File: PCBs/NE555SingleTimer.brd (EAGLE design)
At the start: 22.5 x 32 mm, 5 parts, among them IC1 LM555N

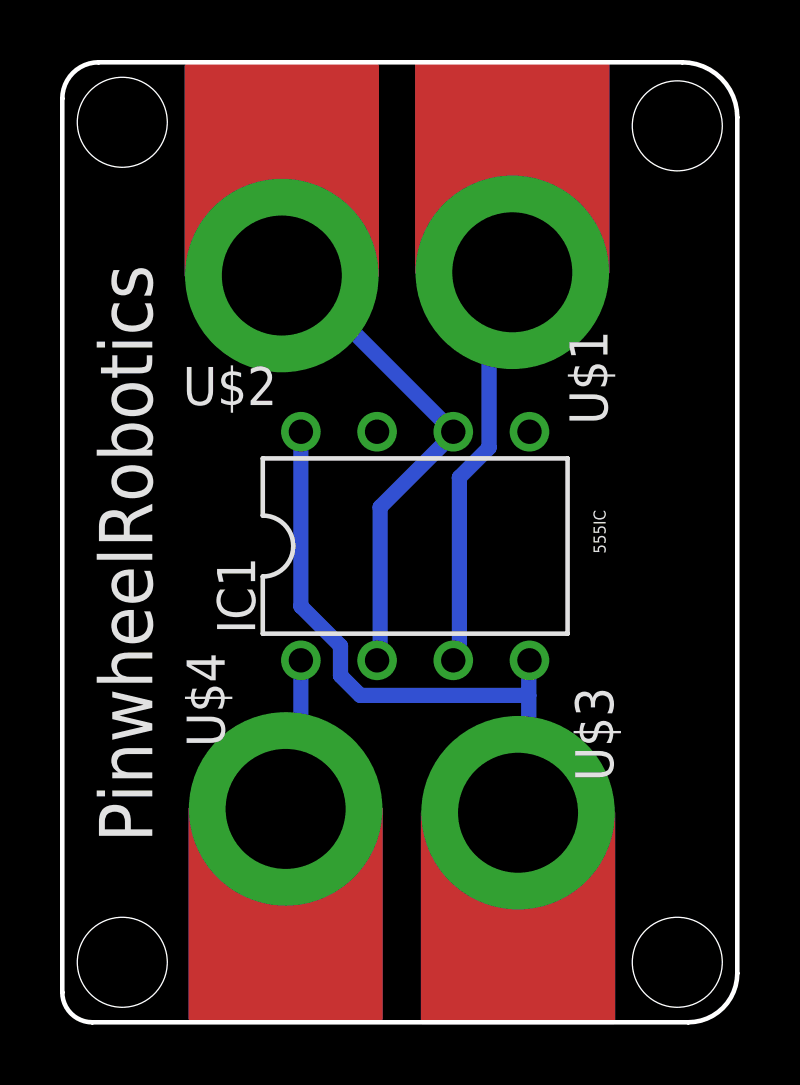
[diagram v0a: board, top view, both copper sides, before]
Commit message: New Update
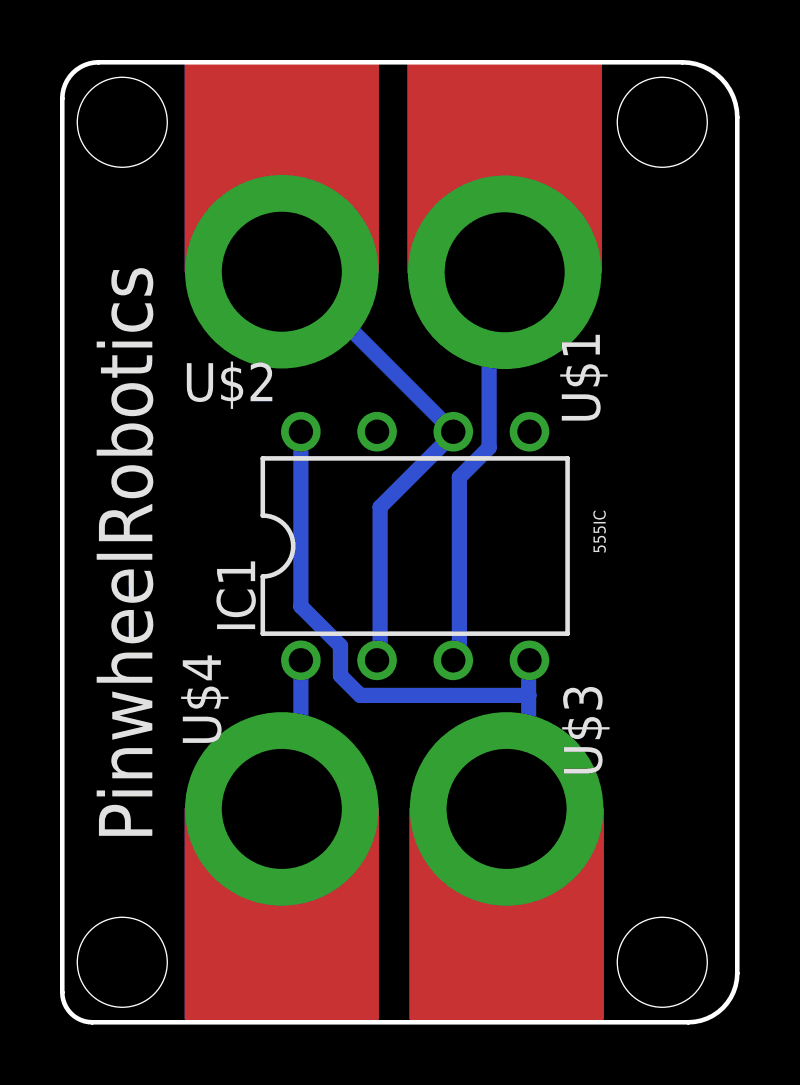
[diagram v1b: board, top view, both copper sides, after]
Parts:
- moved U$3 0.40 mm to (11.8, 7.11)
- moved U$1 0.25 mm to (11.7, 25.0)
- moved U$4 0.13 mm to (4.32, 7.11)
- moved U$2 0.13 mm to (4.32, 25.0)
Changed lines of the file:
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@@
 <drawing>
 <settings>
-<setting alwaysvectorfont="yes"/>
+<setting alwaysvectorfont="no"/>
 <setting verticaltext="up"/>
 </settings>
@@
 <wire x1="-1.788903125" y1="32" x2="-3" y2="30.788903125" width="0.1524" layer="20" curve="90"/>
 <hole x="-1" y="30" drill="3"/>
-<hole x="17.5" y="29.881" drill="3"/>
-<hole x="17.5" y="2" drill="3"/>
+<hole x="17" y="30" drill="3"/>
+<hole x="17" y="2" drill="3"/>
 <hole x="-1" y="2" drill="3"/>
 <text x="0" y="6" size="1.778" layer="21" rot="R90">PinwheelRobotics </text>
@@
 <attribute name="VALUE" x="5.207" y="15.24" size="1.27" layer="27" ratio="10"/>
 </element>
-<element name="U$1" library="microbit" package="MICROBIT_PAD" value="MICROBIT_PAD" x="12" y="25" smashed="yes" rot="R180">
-<attribute name="NAME" x="15.175" y="19.92" size="1.27" layer="21" rot="R90"/>
+<element name="U$1" library="microbit" package="MICROBIT_PAD" value="MICROBIT_PAD" x="11.746" y="25" smashed="yes" rot="R180">
+<attribute name="NAME" x="14.921" y="19.92" size="1.27" layer="21" rot="R90"/>
 </element>
-<element name="U$2" library="microbit" package="MICROBIT_PAD" value="MICROBIT_PAD" x="4.318" y="24.892" smashed="yes" rot="R180">
-<attribute name="NAME" x="1.016" y="20.574" size="1.27" layer="21"/>
+<element name="U$2" library="microbit" package="MICROBIT_PAD" value="MICROBIT_PAD" x="4.318" y="25.019" smashed="yes" rot="R180">
+<attribute name="NAME" x="1.016" y="20.701" size="1.27" layer="21"/>
 </element>
-<element name="U$3" library="microbit" package="MICROBIT_PAD" value="MICROBIT_PAD" x="12.192" y="6.985" smashed="yes">
-<attribute name="NAME" x="14.097" y="11.176" size="1.27" layer="21" rot="R270"/>
+<element name="U$3" library="microbit" package="MICROBIT_PAD" value="MICROBIT_PAD" x="11.811" y="7.112" smashed="yes">
+<attribute name="NAME" x="13.716" y="11.303" size="1.27" layer="21" rot="R270"/>
 </element>
-<element name="U$4" library="microbit" package="MICROBIT_PAD" value="MICROBIT_PAD" x="4.445" y="7.112" smashed="yes">
-<attribute name="NAME" x="1.143" y="12.319" size="1.27" layer="21" rot="R270"/>
+<element name="U$4" library="microbit" package="MICROBIT_PAD" value="MICROBIT_PAD" x="4.318" y="7.112" smashed="yes">
+<attribute name="NAME" x="1.016" y="12.319" size="1.27" layer="21" rot="R270"/>
 </element>
 </elements>
@@
 <wire x1="12.5476" y1="7.5946" x2="12.5476" y2="10.8966" width="0.508" layer="16"/>
 <wire x1="12.5476" y1="10.8966" x2="12.5476" y2="11.8872" width="0.508" layer="16"/>
-<wire x1="12.2428" y1="7.2898" x2="12.5476" y2="7.5946" width="0.508" layer="16"/>
+<wire x1="12.1158" y1="7.1628" x2="12.5476" y2="7.5946" width="0.508" layer="16"/>
 <wire x1="12.5476" y1="11.8872" x2="12.573" y2="12.065" width="0.508" layer="16"/>
-<wire x1="12.2428" y1="7.2898" x2="12.192" y2="6.985" width="0.508" layer="16"/>
+<wire x1="12.1158" y1="7.1628" x2="11.811" y2="7.112" width="0.508" layer="16"/>
 <wire x1="4.953" y1="13.8684" x2="4.953" y2="19.685" width="0.508" layer="16"/>
 <wire x1="6.2738" y1="12.5476" x2="4.953" y2="13.8684" width="0.508" layer="16"/>
@@
 <wire x1="11.2268" y1="19.1516" x2="10.2362" y2="18.161" width="0.508" layer="16"/>
 <wire x1="11.2268" y1="24.1046" x2="11.2268" y2="19.1516" width="0.508" layer="16"/>
-<wire x1="12" y1="24.8778" x2="11.2268" y2="24.1046" width="0.508" layer="16"/>
+<wire x1="11.746" y1="24.6238" x2="11.2268" y2="24.1046" width="0.508" layer="16"/>
 <wire x1="10.2362" y1="12.2174" x2="10.033" y2="12.065" width="0.508" layer="16"/>
-<wire x1="12" y1="24.8778" x2="12" y2="25" width="0.508" layer="16"/>
+<wire x1="11.746" y1="24.6238" x2="11.746" y2="25" width="0.508" layer="16"/>
 </signal>
 <signal name="N$2">
@@
 <wire x1="7.5946" y1="12.2174" x2="7.493" y2="12.065" width="0.508" layer="16"/>
 <wire x1="9.906" y1="19.4818" x2="10.033" y2="19.685" width="0.508" layer="16"/>
-<wire x1="4.826" y1="24.892" x2="10.033" y2="19.685" width="0.508" layer="16"/>
-<wire x1="4.318" y1="24.892" x2="4.826" y2="24.892" width="0.508" layer="16"/>
+<wire x1="4.699" y1="25.019" x2="10.033" y2="19.685" width="0.508" layer="16"/>
+<wire x1="4.318" y1="25.019" x2="4.699" y2="25.019" width="0.508" layer="16"/>
 </signal>
 <signal name="GND">
 <contactref element="IC1" pad="1"/>
 <contactref element="U$4" pad="PAD"/>
-<wire x1="4.953" y1="7.5946" x2="4.953" y2="12.065" width="0.508" layer="16"/>
-<wire x1="4.6228" y1="7.2644" x2="4.953" y2="7.5946" width="0.508" layer="16"/>
-<wire x1="4.6228" y1="7.2644" x2="4.445" y2="7.112" width="0.508" layer="16"/>
+<wire x1="4.953" y1="7.656284375" x2="4.953" y2="12.065" width="0.508" layer="16"/>
+<wire x1="4.953" y1="7.656284375" x2="4.318" y2="7.112" width="0.508" layer="16"/>
 </signal>
 </signals>
